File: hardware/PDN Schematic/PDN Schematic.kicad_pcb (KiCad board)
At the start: 2 copper layers, 59.4 x 69.6 mm, 16 parts, among them J1 Conn_01x02_Pin, J10 Conn_01x02_Pin, J11 Led Indicator Pin, J2 Conn_01x02_Pin, J3 Conn_01x02_Pin, J4 Conn_01x04_Pin, J7 Conn_01x02_Pin, J8 Conn_01x02_Pin, J9 Conn_01x02_Pin, U1 Current Reader

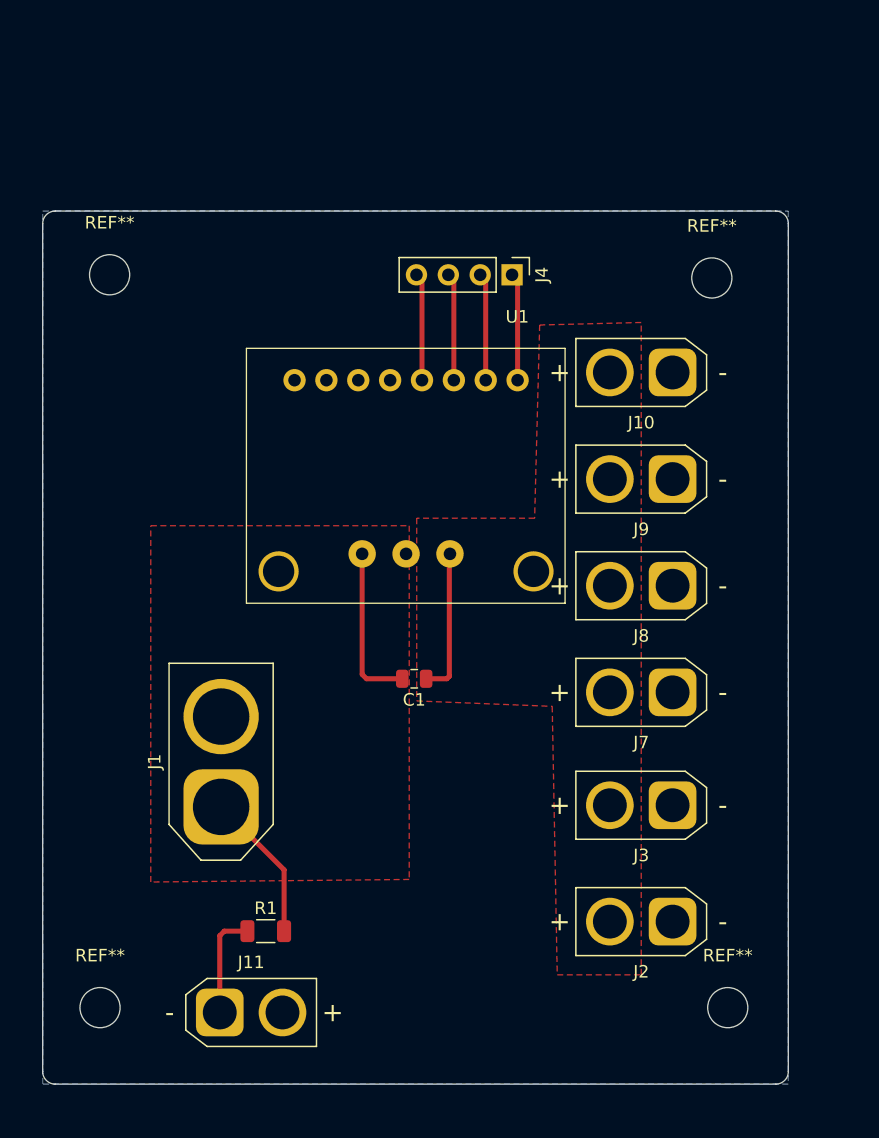
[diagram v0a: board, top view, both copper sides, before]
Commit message: Extra GSE PDN Board changes
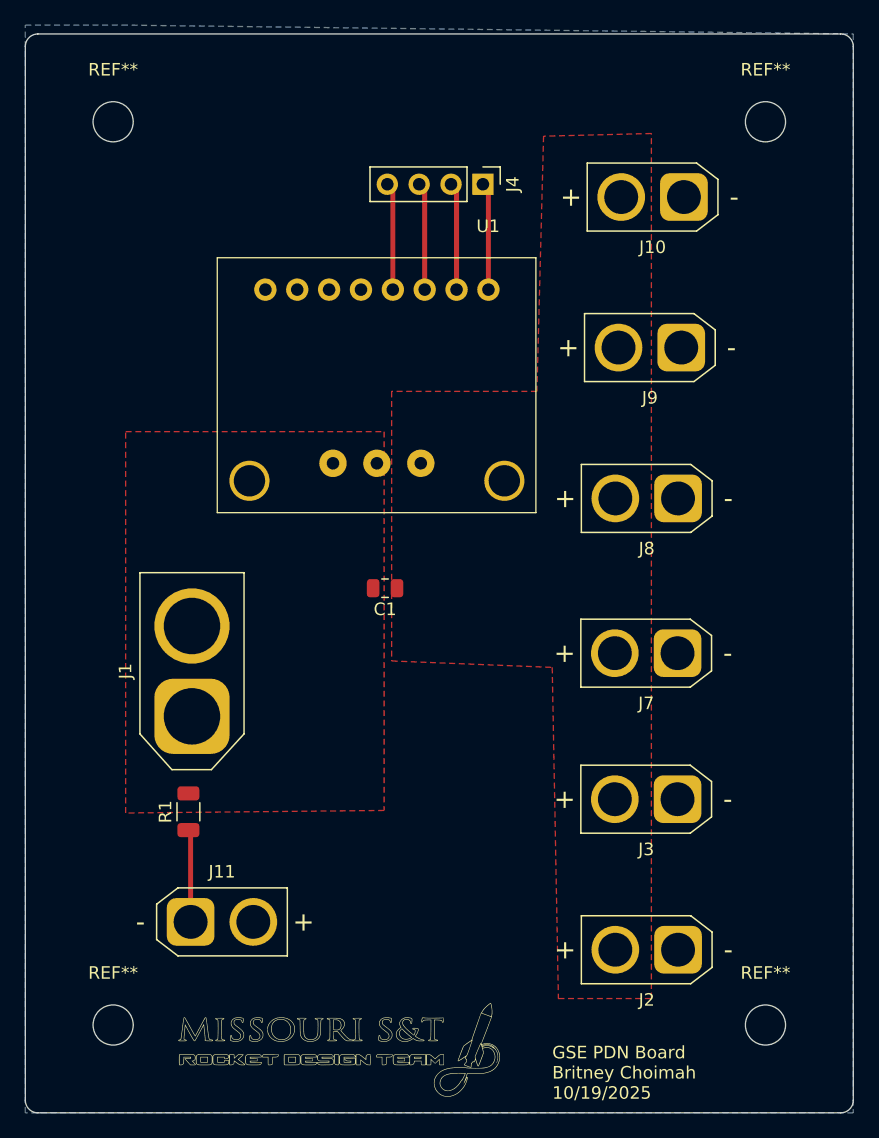
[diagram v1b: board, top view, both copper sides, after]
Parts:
- added G***: LOGO, RDT_Logo:RDT_Logo, F.Cu at (175.0, 106.0)
- moved J10 14.0 mm to (202.5, 38.0)
- moved REF** 13.2 mm to (209.0, 32.0)
- moved REF** 12.2 mm to (157.0, 32.0)
- moved R1 11.3 mm to (163.0, 87.0), turned to 90 degrees
- moved J9 10.5 mm to (202.3, 50.0)
- moved J4 7.58 mm to (186.5, 37.0)
- moved C1 7.58 mm to (178.7, 69.2)
- moved J1 7.58 mm to (163.3, 79.4)
- moved J11 7.58 mm to (163.2, 95.8)
- moved U1 7.58 mm to (186.9, 45.4)
- moved J8 6.97 mm to (202.0, 62.0)
- moved REF** 3.31 mm to (209.0, 104.0)
- moved J7 3.15 mm to (202.0, 74.4)
- moved J2 2.28 mm to (202.0, 98.0)
- moved REF** 1.73 mm to (157.0, 104.0)
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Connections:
- net Net-(J4-Pin_2) renamed GND2
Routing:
- net +13V: track 24.9 -> 0.00 mm
- net VOUT: track 11.5 -> 0.55 mm
- net Net-(J11-Pin_1): track 8.47 -> 7.39 mm
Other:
- board size 59.4 x 69.6 mm -> 66 x 86 mm
- board text added: "GSE PDN Board Britney Choimah 10/19/2025"
